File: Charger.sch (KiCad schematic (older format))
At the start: 42 parts, among them J1 Input, J2 USB-A-S-X-X-SM2, J3 USB-A-S-X-X-SM2, Q1 BSC42DN25NS3, U1 LT1085-5.0, U2 TPS2546, U3 LT3798MPMSETRPBF, U4 TPS2546RTER

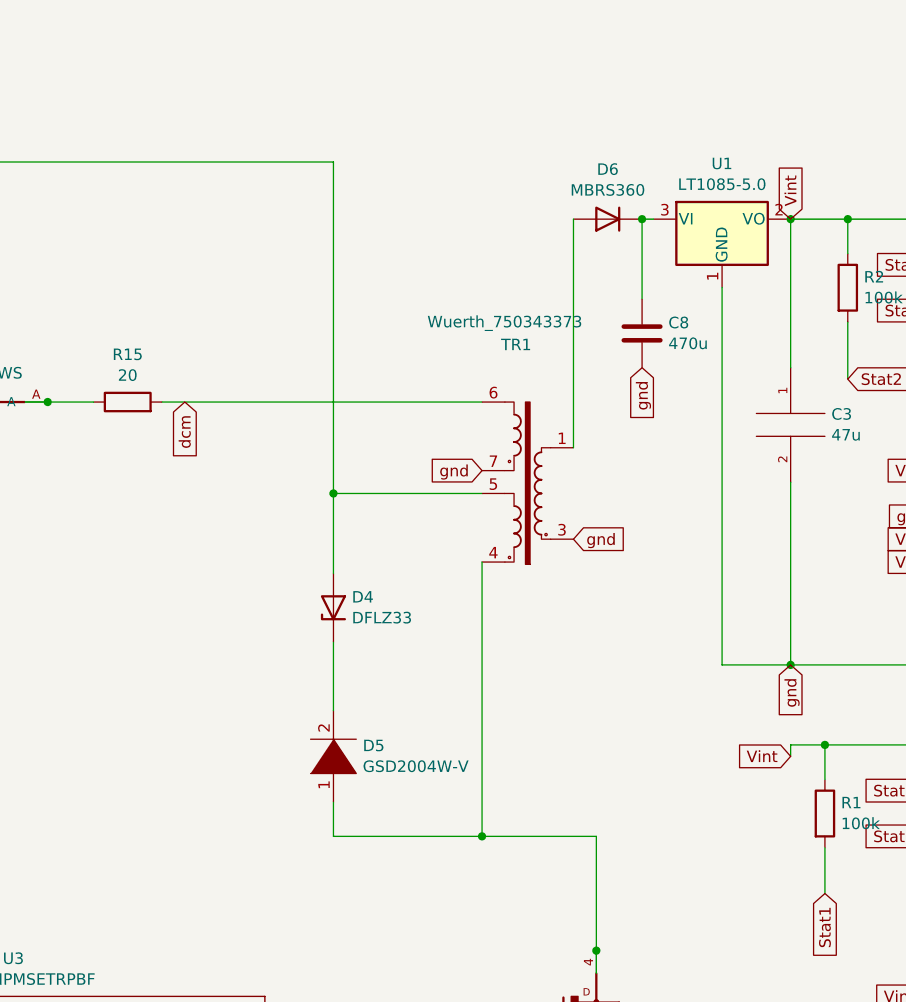
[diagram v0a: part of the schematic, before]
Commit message: transformer footprint added
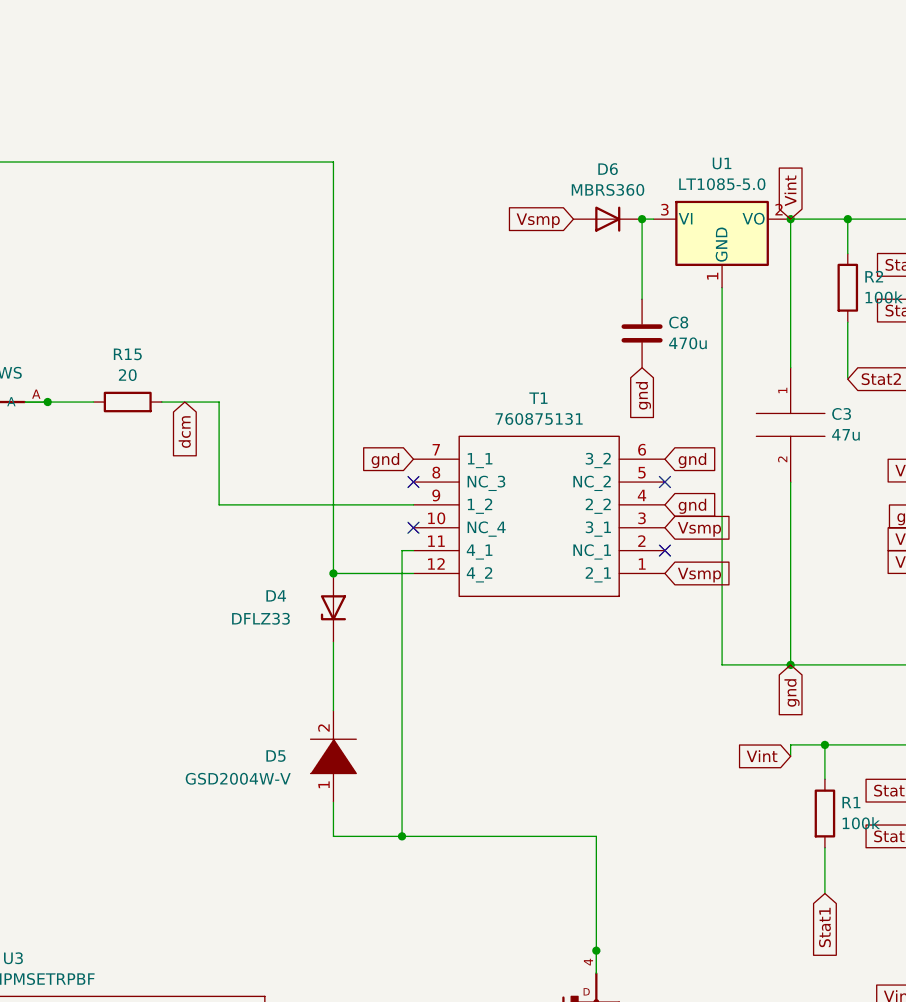
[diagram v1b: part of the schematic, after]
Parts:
- removed TR1: Wuerth_750343373, Transformer_THT:Transformer_Wuerth_750343373, symbol Transformer:Wuerth_750343373
- added T1: 760875131, 760875131:760875131, symbol 760875131:760875131
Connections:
- net labels added: Vsmp
- wire segments 107 -> 108
- no-connect marks 8 -> 12
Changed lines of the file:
@@
 Text GLabel 4600 5950 2    50   Input ~ 0
 gnd
-Wire Wire Line
-	6300 4300 6600 4300
 Connection ~ 6600 4300
 Text GLabel 4600 6050 2    50   Input ~ 0
@@
 U 1 1 603824E5
 P 4600 4700
-F 0 "D5" V 4646 4572 50  0000 R CNN
-F 1 "GSD2004W-V" V 4555 4572 50  0000 R CNN
+F 0 "D5" V 4600 5000 50  0000 R CNN
+F 1 "GSD2004W-V" V 4500 5350 50  0000 R CNN
 F 2 "1N4148WS:SODFL2512X100N" H 4600 4700 50  0001 C CNN
 F 3 "~" H 4600 4700 50  0001 C CNN
@@
 U 1 1 60384E6B
 P 4600 4050
-F 0 "D4" V 4646 3970 50  0000 R CNN
-F 1 "DFLZ33" V 4555 3970 50  0000 R CNN
+F 0 "D4" V 4650 4350 50  0000 R CNN
+F 1 "DFLZ33" V 4550 4500 50  0000 R CNN
 F 2 "1N4148WS:SODFL2512X100N" H 4600 4050 50  0001 C CNN
 F 3 "~" H 4600 4050 50  0001 C CNN
@@
 Wire Wire Line
 	2600 2100 4600 2100
-Wire Wire Line
-	4600 2100 4600 3550
 Connection ~ 2600 2100
-Wire Wire Line
-	4600 5050 5250 5050
-Connection ~ 5250 5050
-Wire Wire Line
-	5250 5050 5750 5050
-Text GLabel 5250 3450 0    50   Input ~ 0
-gnd
 Text GLabel 3950 3150 3    50   Input ~ 0
 dcm
@@
 	5950 2350 6000 2350
 Connection ~ 5950 2350
-Wire Wire Line
-	5650 2350 5650 3350
 Text GLabel 5950 3000 3    50   Input ~ 0
 gnd
@@
 	2750 3150 2950 3150
 $Comp
-L Transformer:Wuerth_750343373 TR1
-U 1 1 603B20C8
-P 5450 3550
-F 0 "TR1" H 5500 2900 50  0000 C CNN
-F 1 "Wuerth_750343373" H 5550 2800 50  0000 C CNN
-F 2 "Transformer_THT:Transformer_Wuerth_750343373" H 5450 3000 50  0001 C CNN
-F 3 "https://katalog.we-online.com/ctm/datasheet/750343373.pdf" H 5450 3550 50  0001 C CNN
-	1    5450 3550
-	-1   0    0    1
-$EndComp
-Wire Wire Line
-	3850 3150 5250 3150
-Wire Wire Line
-	5250 3550 4600 3550
-Connection ~ 4600 3550
-Wire Wire Line
-	4600 3550 4600 3900
-Wire Wire Line
-	5250 3850 5250 5050
-Text GLabel 5650 3750 2    50   Input ~ 0
-gnd
-$Comp
 L FQT4N25TF:FQT4N25TF Q1
 U 1 1 603D4489
@@
 Wire Wire Line
 	5750 5550 5750 5650
+Text GLabel 5650 2350 0    50   Input ~ 0
+Vsmp
+$Comp
+L 760875131:760875131 T1
+U 1 1 60386D1D
+P 6050 3900
+F 0 "T1" H 6600 3135 50  0000 C CNN
+F 1 "760875131" H 6600 3226 50  0000 C CNN
+F 2 "760875131:760875131" H 7000 4000 50  0001 L CNN
+F 3 "https://katalog.we-online.de/pbs/datasheet/760875131.pdf" H 7000 3900 50  0001 L CNN
+F 4 "Audio Transformers / Signal Transformers WE-UOST Univ Offline 1500uH 0.8A 140mOhm" H 7000 3800 50  0001 L CNN "Description"
+F 5 "14" H 7000 3700 50  0001 L CNN "Height"
+F 6 "Wurth Elektronik" H 7000 3600 50  0001 L CNN "Manufacturer_Name"
+F 7 "760875131" H 7000 3500 50  0001 L CNN "Manufacturer_Part_Number"
+F 8 "710-760875131" H 7000 3400 50  0001 L CNN "Mouser Part Number"
+F 9 "https://www.mouser.co.uk/ProductDetail/Wurth-Elektronik/760875131?qs=TB%2FQ0sBK%2FGdsHNIF9xNITw%3D%3D" H 7000 3300 50  0001 L CNN "Mouser Price/Stock"
+F 10 "" H 7000 3200 50  0001 L CNN "Arrow Part Number"
+F 11 "" H 7000 3100 50  0001 L CNN "Arrow Price/Stock"
+	1    6050 3900
+	-1   0    0    1
+$EndComp
+Wire Wire Line
+	4600 2100 4600 3900
+Wire Wire Line
+	4600 5050 4900 5050
+Wire Wire Line
+	6300 4300 6600 4300
+Text GLabel 6050 3600 2    50   Input ~ 0
+gnd
+Text GLabel 6050 3400 2    50   Input ~ 0
+gnd
+Wire Wire Line
+	3850 3150 4100 3150
+Wire Wire Line
+	4100 3150 4100 3600
+Wire Wire Line
+	4100 3600 4950 3600
+Text GLabel 4950 3400 0    50   Input ~ 0
+gnd
+Wire Wire Line
+	4950 3900 4600 3900
+Connection ~ 4600 3900
+Wire Wire Line
+	4950 3800 4900 3800
+Wire Wire Line
+	4900 3800 4900 5050
+Connection ~ 4900 5050
+Wire Wire Line
+	4900 5050 5750 5050
+Text GLabel 6050 3900 2    50   Input ~ 0
+Vsmp
+Text GLabel 6050 3700 2    50   Input ~ 0
+Vsmp
+NoConn ~ 4950 3500
+NoConn ~ 4950 3700
+NoConn ~ 6050 3800
+NoConn ~ 6050 3500
 $EndSCHEMATC
